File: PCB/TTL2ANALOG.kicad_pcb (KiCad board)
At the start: 2 copper layers, 60.5 x 56.1 mm, 39 parts, among them J1 EGA/CGA, J2 Brown Fix, J3 CSync Inv., J4 Sync Type, J5 TTL Input, J6 Analog Out, J7 Barrel_Jack, U1 GAL20V8, U2 74LS244, U3 74LS244, U4 L7805

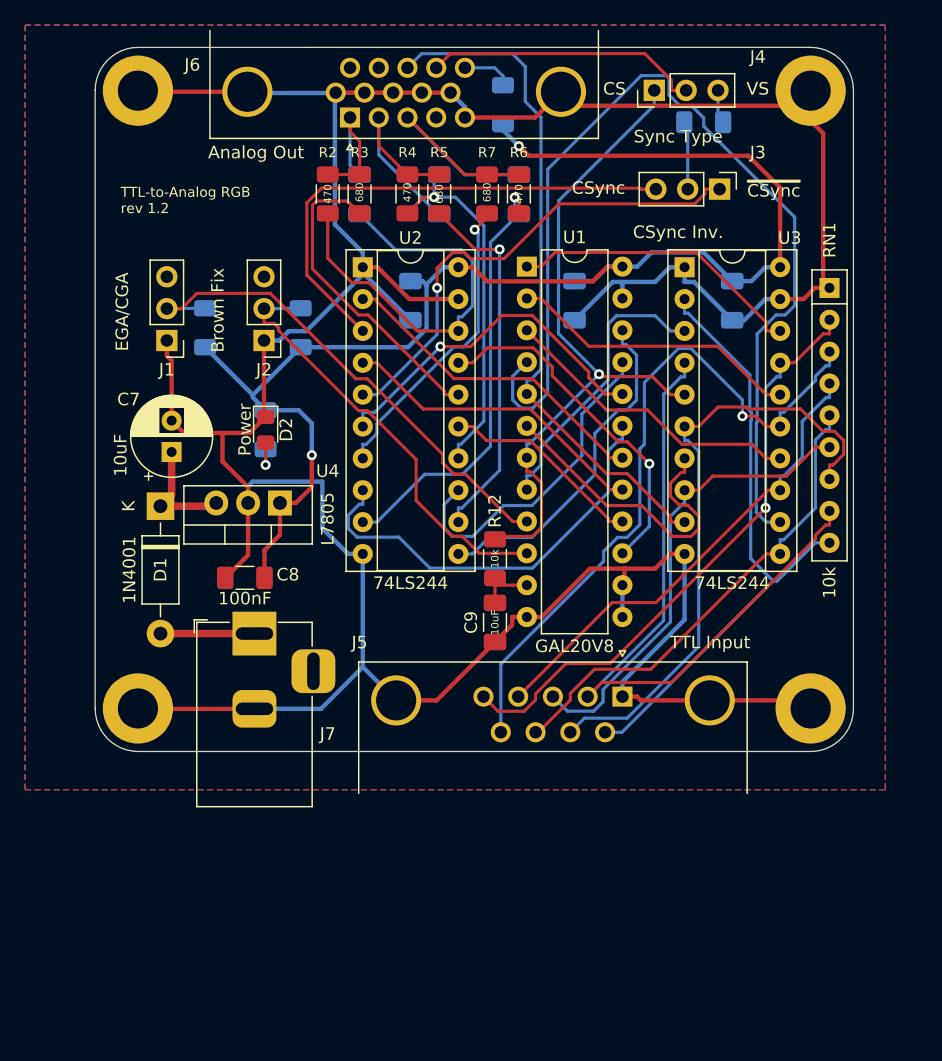
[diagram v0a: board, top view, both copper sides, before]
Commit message: Redraw version 1.4
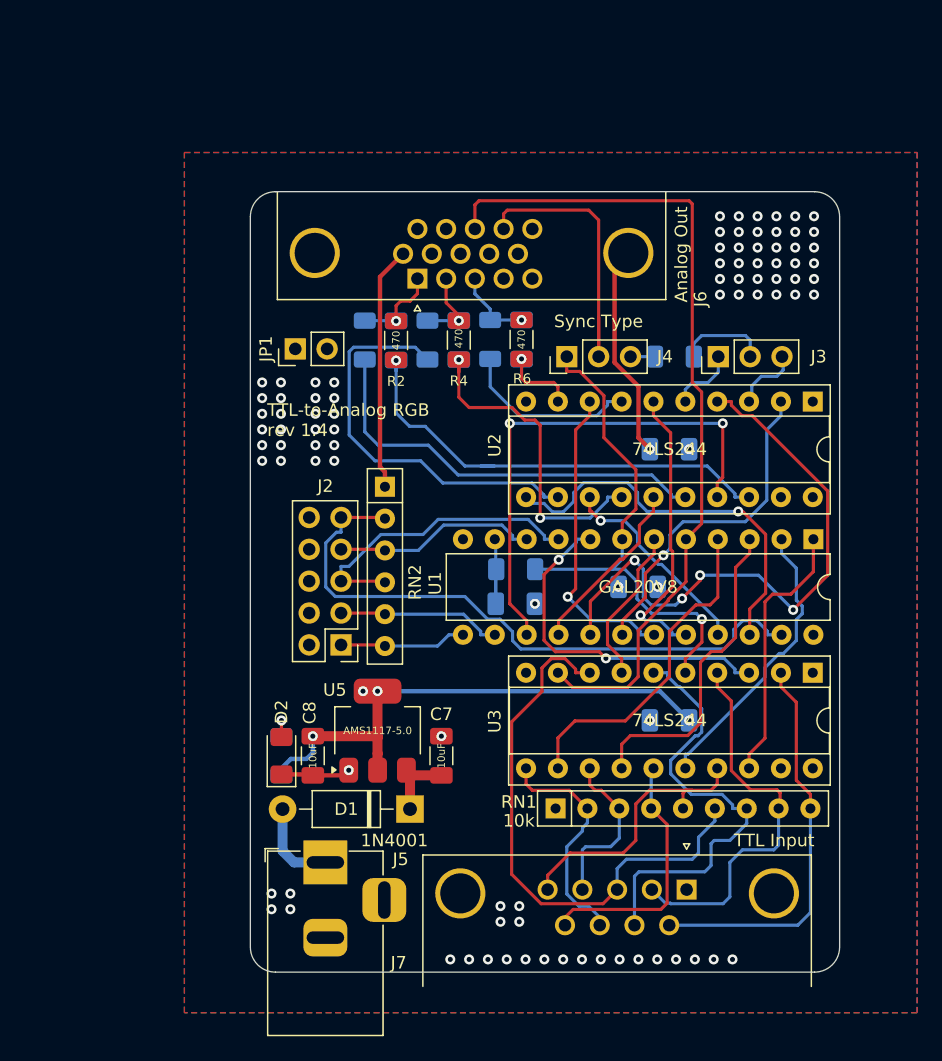
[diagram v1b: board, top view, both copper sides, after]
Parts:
- removed H1, H2, H3, H4: MountingHole_Pad, MountingHole:MountingHole_3.2mm_M3_DIN965_Pad
- removed J1: EGA/CGA, Connector_PinHeader_2.54mm:PinHeader_1x03_P2.54mm_Vertical
- removed R13: 0, Resistor_SMD:R_1206_3216Metric_Pad1.30x1.75mm_HandSolder
- removed R8, R9: 10k, Resistor_SMD:R_1206_3216Metric_Pad1.30x1.75mm_HandSolder
- removed U4: L7805, Package_TO_SOT_THT:TO-220-3_Vertical
- added JP1: 5V on video, Connector_PinHeader_2.54mm:PinHeader_1x02_P2.54mm_Vertical, F.Cu at (123.1, 74.1)
- added RN2: 10k, Resistor_THT:R_Array_SIP6, F.Cu at (130.3, 85.1)
- added U5: AMS1117-5.0, Package_TO_SOT_SMD:SOT-223-3_TabPin2, F.Cu at (129.7, 104.5)
- C7: footprint Capacitor_THT:CP_Radial_D6.3mm_P2.50mm -> Capacitor_SMD:C_1206_3216Metric_Pad1.33x1.80mm_HandSolder
- C8: value 100nF -> 10uF
- C9, R12, R3, R5, R7: moved to B.Cu
- D2: footprint LED_SMD:LED_0805_2012Metric_Pad1.15x1.40mm_HandSolder -> LED_SMD:LED_1206_3216Metric_Pad1.42x1.75mm_HandSolder
- J2: value Brown Fix -> Options; footprint Connector_PinHeader_2.54mm:PinHeader_1x03_P2.54mm_Vertical -> Connector_PinHeader_2.54mm:PinHeader_2x05_P2.54mm_Vertical
- moved RN1 46.9 mm to (143.9, 110.7), turned to 0 degrees
- moved U2 37.4 mm to (164.4, 78.3), turned to -90 degrees
- moved U3 33.9 mm to (164.4, 99.9), turned to -90 degrees
- moved C5 33.8 mm to (153.0, 103.7), turned to 180 degrees
- moved C7 32.4 mm to (134.8, 106.5)
- moved U1 31.5 mm to (164.4, 89.2), turned to -90 degrees
- moved D1 31.3 mm to (132.3, 110.8), turned to 180 degrees
- moved D2 26.0 mm to (122.0, 106.5), turned to 90 degrees
- moved R11 26.0 mm to (122.0, 106.5), turned to -90 degrees
- moved J2 25.0 mm to (126.8, 97.7)
- moved C6 23.8 mm to (153.0, 82.1), turned to 180 degrees
- moved C4 23.4 mm to (150.5, 93.0), turned to 180 degrees
- moved J4 22.3 mm to (144.8, 74.7)
- moved J7 19.1 mm to (125.5, 115.0)
- moved R10 18.8 mm to (153.4, 74.7), turned to 180 degrees
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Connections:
- J2 pad 1: GND -> Net-(J2-Pin_1)
- J2 pad 2: /BRWN_FIX -> VCC
- J2 pad 3: (no net) -> Net-(J2-Pin_3)
- J6 pad 11: (no net) -> unconnected-(J6-Pad11)
- J6 pad 12: (no net) -> unconnected-(J6-Pad12)
- J6 pad 15: Net-(J6-Pad15) -> unconnected-(J6-Pad15)
- J6 pad 4: (no net) -> unconnected-(J6-Pad4)
- J6 pad 9: GND -> Net-(JP1-B)
- RN1 pad 2: /IN_B -> /IN_HS
- RN1 pad 3: /IN_VS -> /IN_G
- RN1 pad 4: /IN_G -> /IN_VS
- RN1 pad 5: /IN_HS -> /IN_B
- U1 pad 13: GND -> Net-(J2-Pin_1)
- U1 pad 14: GND -> Net-(J2-Pin_3)
- U1 pad 23: GND -> Net-(J2-Pin_9)
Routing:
- net GND: track 281.2 -> 413.0 mm, vias 0 -> 90
- net /IN_R_BUF: track 81.0 -> 26.6 mm
- net Net-(J2-Pin_9): track 0.00 -> 50.6 mm
- net Net-(JP1-B): track 0.00 -> 35.5 mm
- net /IN_VS: track 56.3 -> 20.9 mm, vias 1 -> 0
- net /~{OUT_CS}: track 40.4 -> 5.48 mm
- net /OUT_CS: track 38.9 -> 6.02 mm, vias 1 -> 0
- net /OUT_B: track 35.0 -> 5.92 mm
- net VCC: track 113.4 -> 139.3 mm, vias 2 -> 6
- net /IN_B: track 48.2 -> 22.7 mm, vias 1 -> 0
- net /IN_R_I: track 56.2 -> 31.2 mm
- net /IN_G: track 38.3 -> 13.3 mm
- net /DEC_R_I: track 25.0 -> 47.9 mm, vias 0 -> 4
- net /IN_HS: track 38.7 -> 18.5 mm
- net /BRWN_FIX: track 34.7 -> 16.3 mm
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- added copper zone on In1.Cu, net GND
- added copper zone on In2.Cu, net VCC
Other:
- board size 60.5 x 56.1 mm -> 47 x 62.2 mm
- copper layers 2 -> 4
- board text added: "TTL-to-Analog RGB rev 1.4"
- board text removed: "CS"
- board text removed: "CSync"
- board text removed: "TTL-to-Analog RGB rev 1.2"
- board text removed: "VS"
- board text removed: "~{CSync}"
- board text removed: "~{SYNC}"
